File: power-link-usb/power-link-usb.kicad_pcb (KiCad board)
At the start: 4 copper layers, 60 x 30 mm, 35 parts, among them J101 NE8FAH, J102 NE8FAH, J103 DX07S016JA3, Q101 BSC010N04LS, Q102 BSC010N04LS, U101 CYPD3176-24LQ

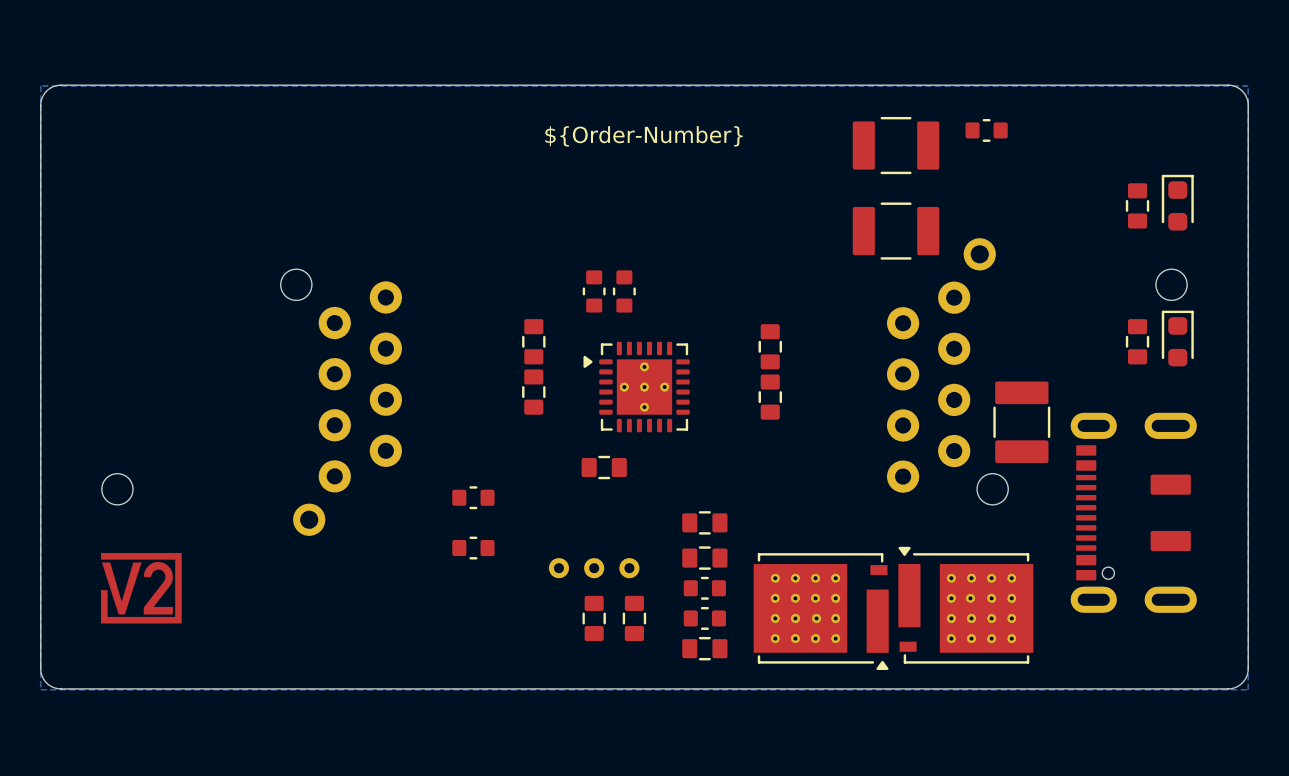
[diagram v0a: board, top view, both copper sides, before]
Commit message: Fix WAGOs
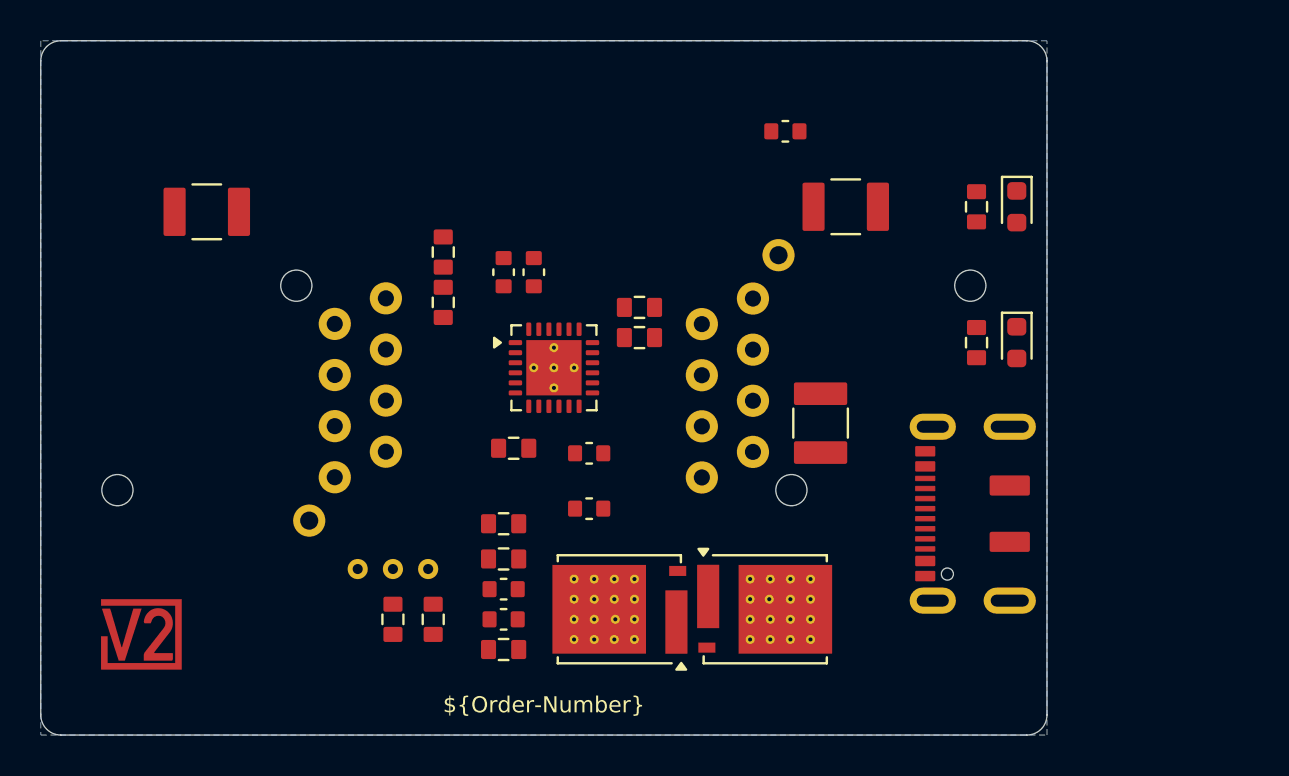
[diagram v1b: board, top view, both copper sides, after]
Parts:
- removed R111: 5k1, V2_Resistor_SMD:R_0603
- removed R112: 1k, V2_Resistor_SMD:R_0603
- added R114: 5k1, V2_Resistor_SMD:R_0603, F.Cu at (146.8, 95.8)
- added R115: 1k, V2_Resistor_SMD:R_0603, F.Cu at (146.8, 97.2)
- moved C105 34.4 mm to (125.2, 91.0)
- moved INFO101 28.7 mm to (142.0, 115.5)
- moved C101 10.0 mm to (140.0, 109.8)
- moved C102 10.0 mm to (140.0, 111.2)
- moved C107 10.0 mm to (154.0, 87.0)
- moved J102 10.0 mm to (167.0, 99.8)
- moved Q101 10.0 mm to (153.0, 110.8)
- moved Q102 10.0 mm to (145.8, 110.8)
- moved R101 10.0 mm to (140.0, 108.2)
- moved R102 10.0 mm to (140.0, 106.5)
- moved R103 10.0 mm to (140.0, 112.8)
- moved R109 10.0 mm to (136.5, 111.2)
- moved R110 10.0 mm to (134.5, 111.2)
- moved R113 10.0 mm to (155.8, 101.5)
- moved TP101 10.0 mm to (136.2, 108.8)
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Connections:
- U101 pad 16: /Current-Min -> PGND
- U101 pad 17: PGND -> /Current-Min
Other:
- board size 60 x 30 mm -> 50 x 34.5 mm
